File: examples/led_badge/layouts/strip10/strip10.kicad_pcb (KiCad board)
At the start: 2 copper layers, 20 parts

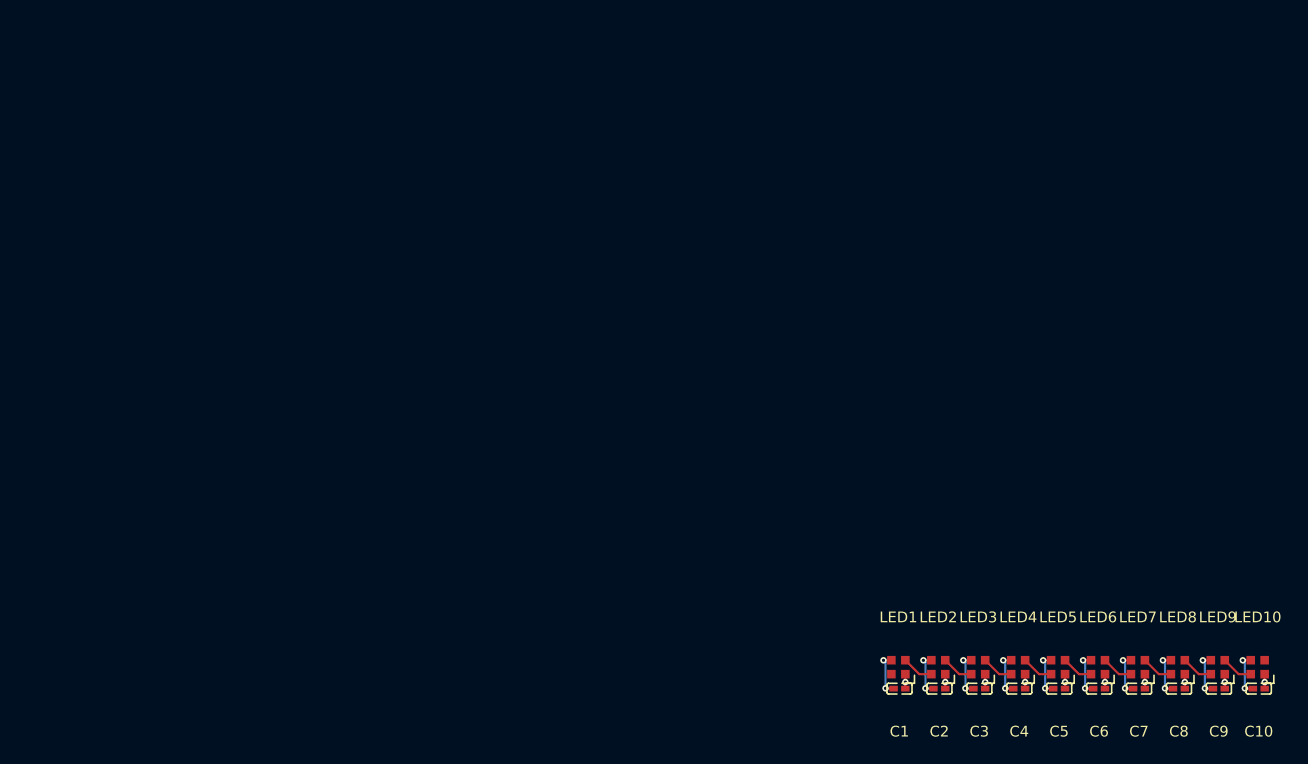
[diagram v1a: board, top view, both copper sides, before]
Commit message: rebuild lad badge
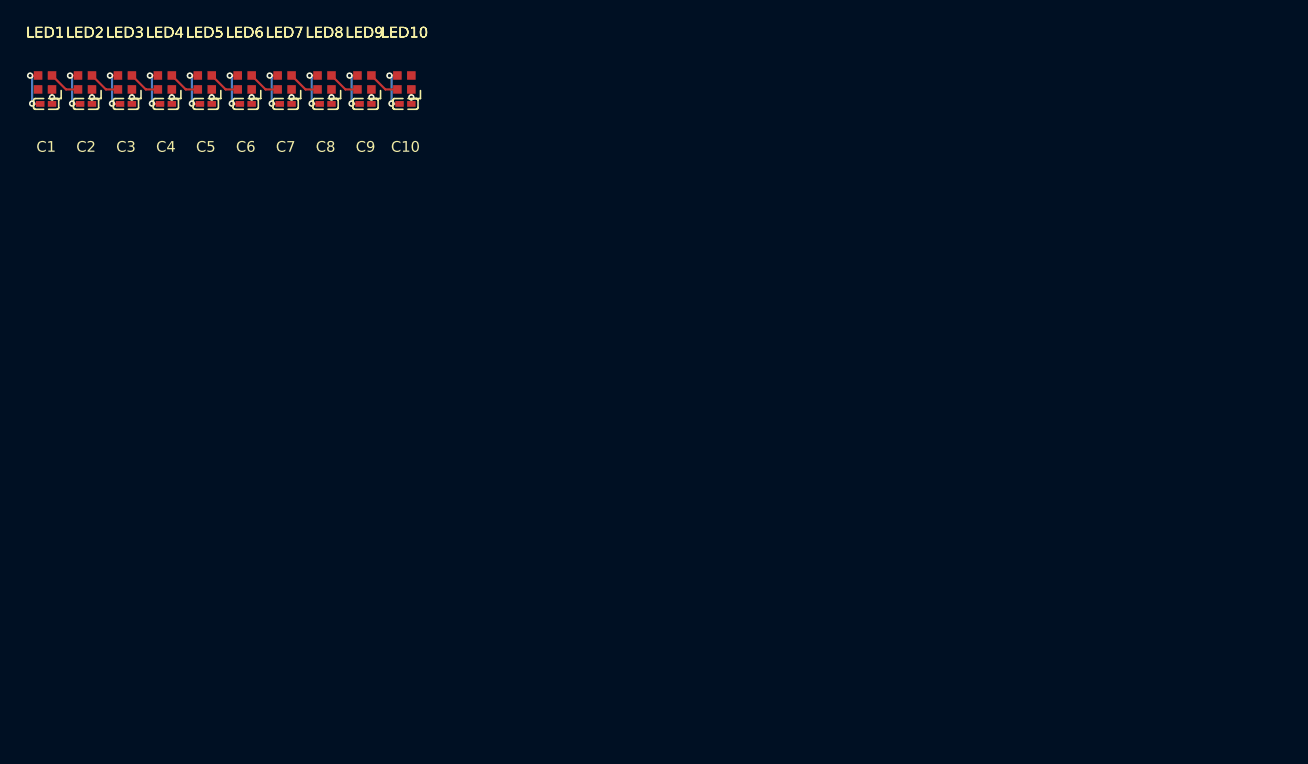
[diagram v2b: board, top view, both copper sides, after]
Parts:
- C1, C10, C2, C3, C4, C5, C6, C7, C8, C9: value 100nF ±10% 16V X7R -> 100nF ±10% 50V X7R; footprint Samsung_Electro_Mechanics_CL05B104KO5NNNC:C0402 -> Samsung_Electro_Mechanics_CL05B104KB54PNC:C0402
- moved C1 96.4 mm to (61.0, 46.2)
- moved C4 96.4 mm to (72.1, 46.2)
- moved C5 96.4 mm to (75.9, 46.2)
- moved C8 96.4 mm to (87.0, 46.2)
- moved C9 96.4 mm to (90.8, 46.2)
- moved LED3 96.4 mm to (68.3, 44.2)
- moved LED4 96.4 mm to (72.0, 44.2)
- moved LED7 96.4 mm to (83.2, 44.2)
- moved LED8 96.4 mm to (86.9, 44.2)
- moved C10 96.4 mm to (94.5, 46.2)
- moved C2 96.4 mm to (64.7, 46.2)
- moved C3 96.4 mm to (68.4, 46.2)
- moved C6 96.4 mm to (79.6, 46.2)
- moved C7 96.4 mm to (83.3, 46.2)
- moved LED1 96.4 mm to (60.9, 44.2)
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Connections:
- net -DOUT-0 renamed DOUT
- net -DOUT-1 renamed leds[1]-data_in-DIN
- net -DOUT-2 renamed leds[2]-data_in-DIN
- net -DOUT-3 renamed leds[3]-data_in-DIN
- net -DOUT-4 renamed leds[4]-data_in-DIN
- net -DOUT-5 renamed leds[5]-data_in-DIN
- net -DOUT-6 renamed leds[6]-data_in-DIN
- net -DOUT-7 renamed leds[7]-data_in-DIN
- net -DOUT-8 renamed leds[8]-data_in-DIN
- net -DOUT-9 renamed leds[9]-data_in-DIN
- net DIN renamed leds[0]-data_in-DIN
- net gnd renamed GND
- net hv renamed VCC
